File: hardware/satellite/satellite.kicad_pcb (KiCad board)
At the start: 4 copper layers, 17 x 35 mm, 24 parts, among them J1 CHAIN IN, J2 CHAIN OUT, J3 ICE / INITIAL FLASH, J4 PROTECTED CELL 90mAh, J5 NTC (optional), M1 VLV041235L, U1 M2003FC1AE, U2 DRV2625

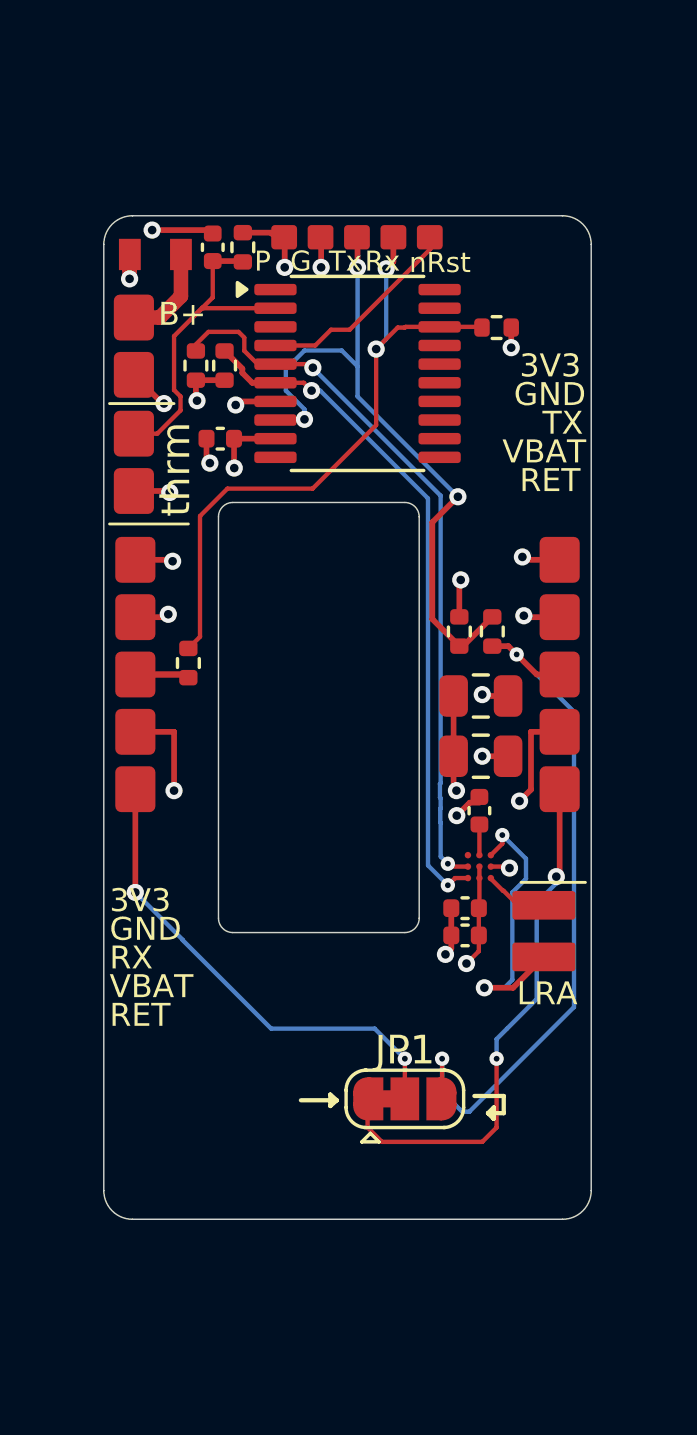
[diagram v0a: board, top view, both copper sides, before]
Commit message: PCB housing
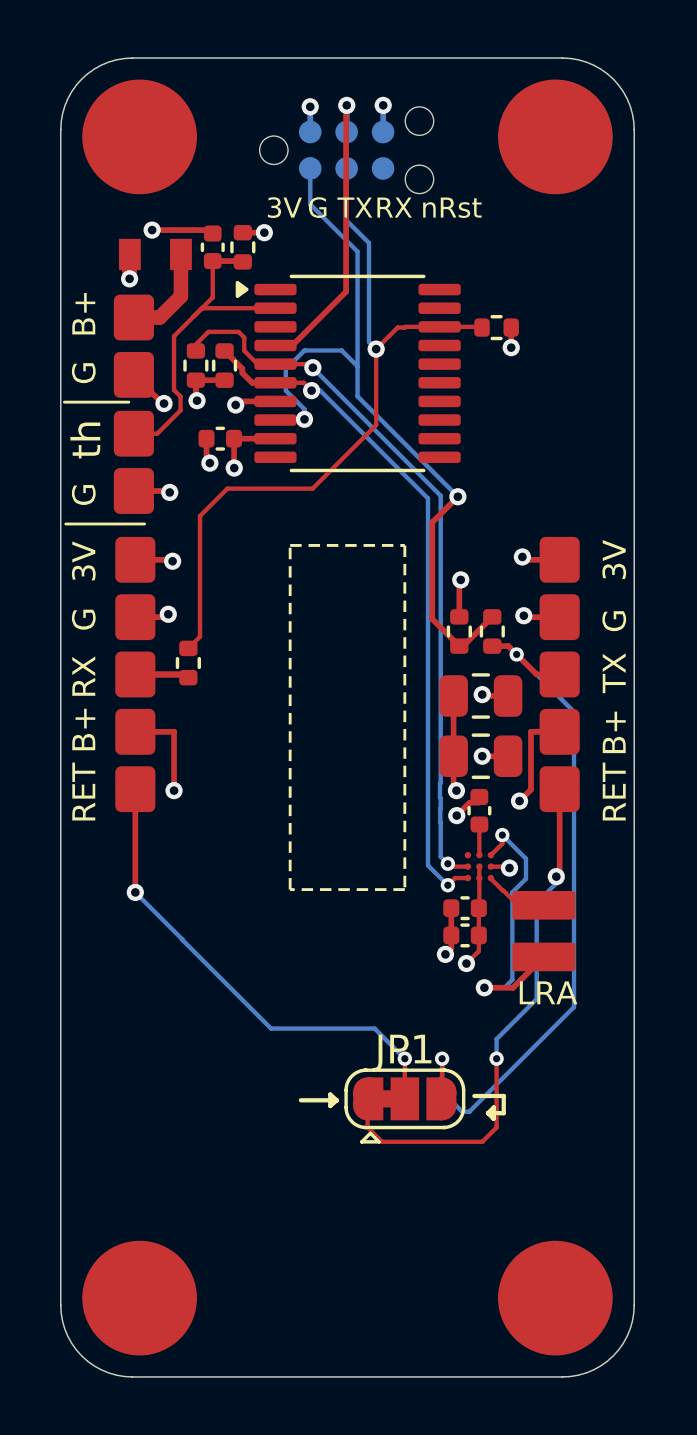
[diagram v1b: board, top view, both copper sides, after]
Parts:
- removed J3: ICE / INITIAL FLASH, HapticBracelet:WirePads_5_P1.27mm
- added H1: M1.6 STANDOFF, HapticBracelet:SMT_Standoff_M1p6_D3p3_ClosedBase_HeightTBD, F.Cu at (104.2, 93.2)
- added H2: M1.6 STANDOFF, HapticBracelet:SMT_Standoff_M1p6_D3p3_ClosedBase_HeightTBD, F.Cu at (118.8, 93.2)
- added H3: M1.6 STANDOFF, HapticBracelet:SMT_Standoff_M1p6_D3p3_ClosedBase_HeightTBD, F.Cu at (104.2, 133.8)
- added H4: M1.6 STANDOFF, HapticBracelet:SMT_Standoff_M1p6_D3p3_ClosedBase_HeightTBD, F.Cu at (118.8, 133.8)
- added J6: Conn_ARM_SWD_TagConnect_TC2030-NL, Connector:Tag-Connect_TC2030-IDC-NL_2x03_P1.27mm_Vertical, B.Cu at (111.5, 93.7)
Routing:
- net /LOCAL_nRESET: track 7.11 -> 10.4 mm, vias 0 -> 1
- net /UART_TX_LOCAL: track 24.0 -> 27.2 mm, vias 3 -> 2
- net /UART_RX_LOCAL: track 22.8 -> 25.6 mm, vias 2 -> 1
- net +3V3_POD: track 16.8 -> 15.9 mm, vias 10 -> 11
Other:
- board size 17 x 35 mm -> 20 x 46 mm
- board text added: "20 x 46 mm POD FACE / R2.5 Cmts.User: TPU contact inner edge, 1.2 mm inset Dwgs.User dashed: placement limit, 1.5 mm inset Corner circles: D4.6 TPU standoff relief Height / screw length TBD; drawings are not copper keepouts"
- board text added: "3V"
- board text added: "Dashed 4 x 12: LRA body proposal; factory tape M1 flex-contact placement remains to be adjusted"
- board text added: "th"
- board text removed: "3V3"
- board text removed: "GND"
- board text removed: "P"
- board text removed: "Rx"
- board text removed: "Tx"
- board text removed: "VBAT"
- board text removed: "thrm"
